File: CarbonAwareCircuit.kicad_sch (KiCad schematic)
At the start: 12 parts, among them J1 USB_C_Receptacle_USB2.0_14P, SW1 SW_Push, U1 LD1117V, U2 ESP32-C3-WROOM-02

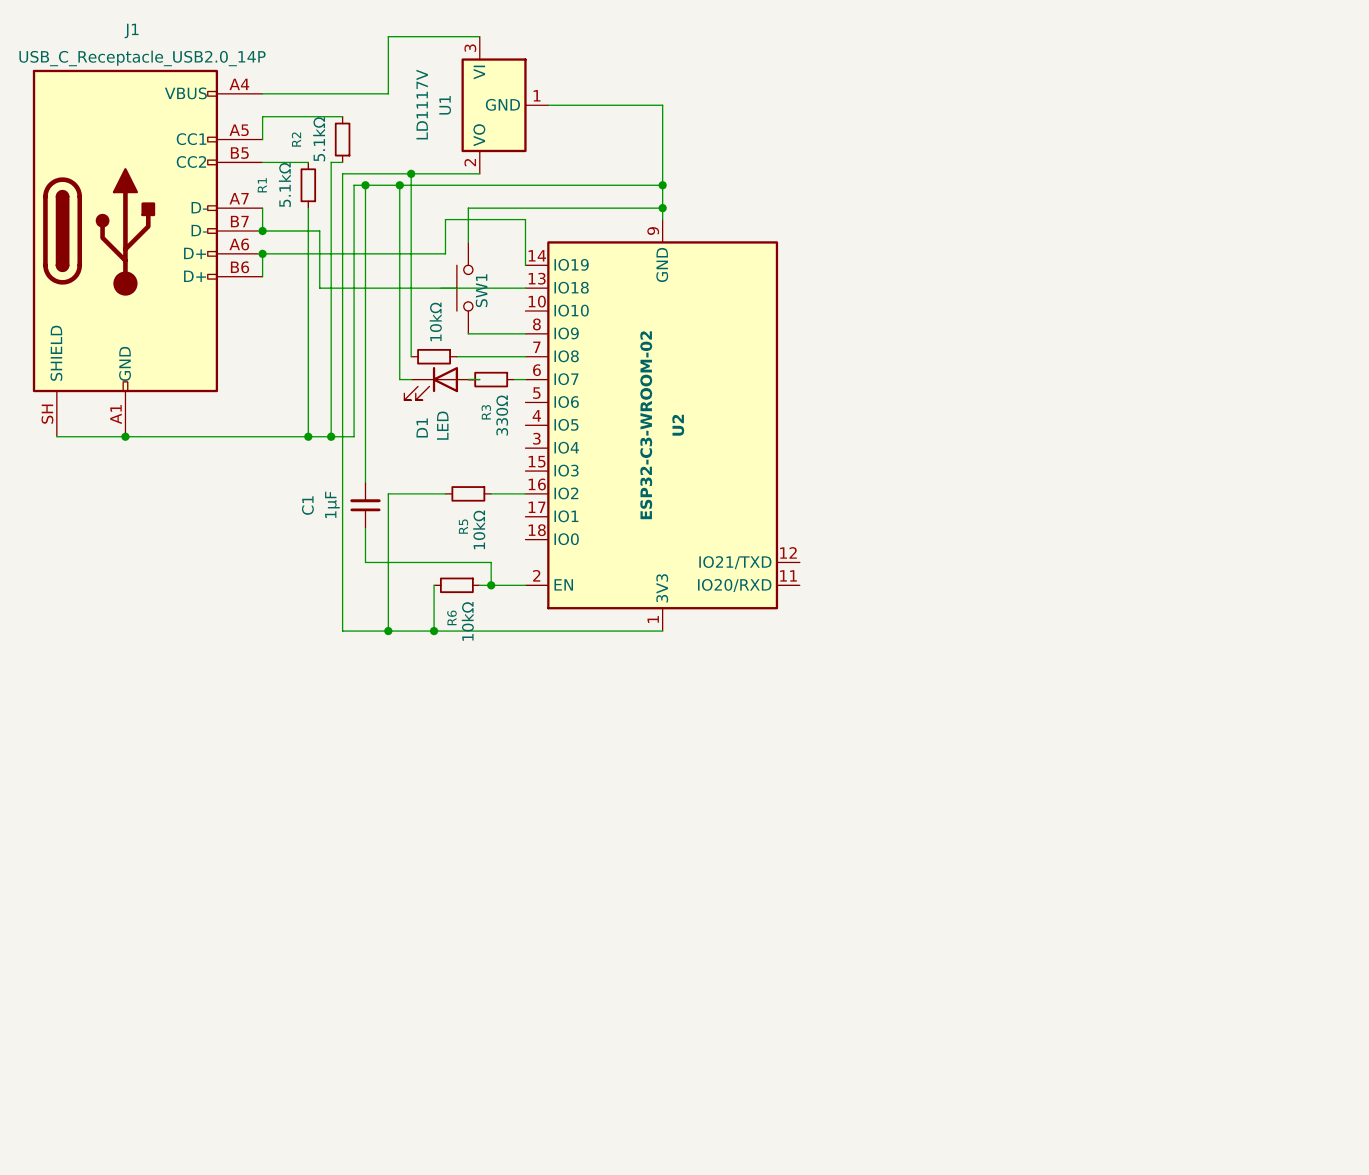
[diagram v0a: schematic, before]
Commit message: eeschema done
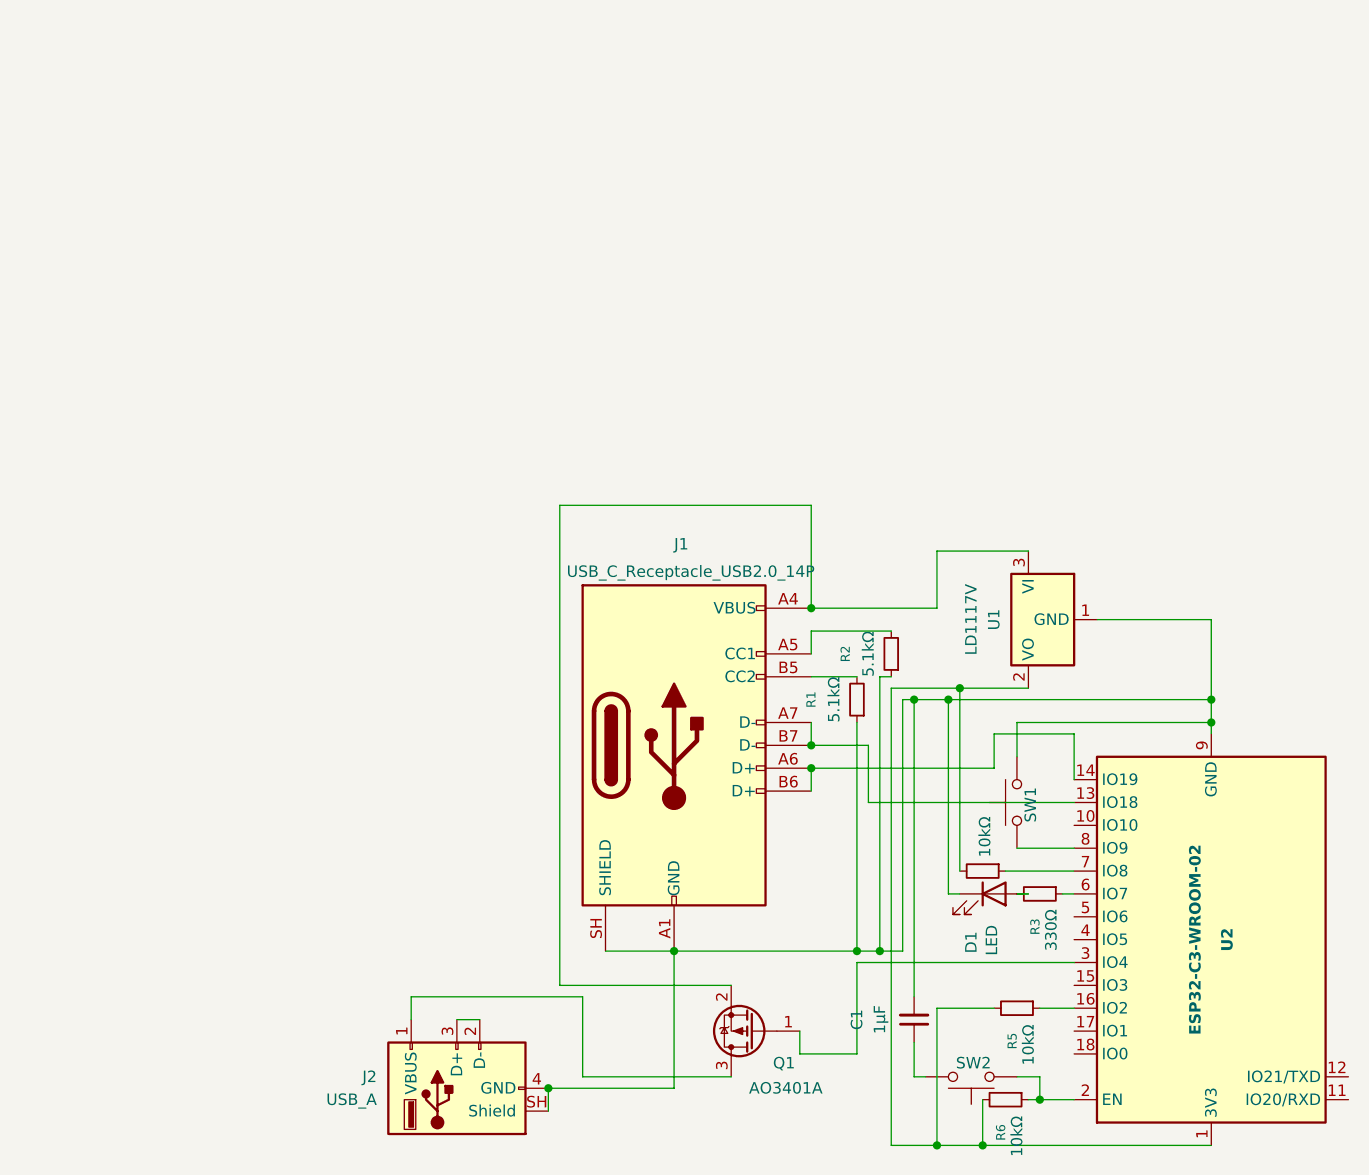
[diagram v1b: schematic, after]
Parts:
- added J2: USB_A, symbol Connector:USB_A
- added Q1: AO3401A, Package_TO_SOT_SMD:SOT-23, symbol Transistor_FET:AO3401A
- added SW2: SW_Push, symbol Switch:SW_Push
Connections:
- net at C1.2, D1.1 (K), J1.A1 (GND)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: now also J2.4 (GND), J2.SH (Shield)
- net at R6.1, U2.2 (EN): now also SW2.1; no longer C1.1
- net at U2.3 (IO4): now also Q1.1 (G)
- net at J1.A4 (VBUS), J1.A9 (VBUS), J1.B4 (VBUS)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: now also Q1.2 (S)
- new net: C1.1, SW2.2
- new net: J2.1 (VBUS), Q1.3 (D)
- new net: J2.2 (D-), J2.3 (D+)
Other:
- moved on the sheet: C1, D1, J1, R1, R2, R3, R5, R6, SW1, U1, U2
